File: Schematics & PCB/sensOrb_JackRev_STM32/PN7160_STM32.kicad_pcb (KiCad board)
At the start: 4 copper layers, 56.2 x 56.2 mm, 87 parts, among them J1 USB4215-03-A_REVA, J10 Conn_01x02, J11 STM32 Optional I/O, J12 Antenna_Conn, J2 Conn_01x04, J3 Conn_01x04, J4 Conn_01x04, J5 Conn_01x04, J6 Conn_01x04, J7 Conn_01x04, J8 IMU Top, J9 IMU Bottom, SW1 SW_SPST, SW2 SW_SPST, U1 PN7160A1HN/C100E, U3 STM32F411CEU6, U4 TLV75533PDBVR, U5 TPS61070DDCR, U6 TCA9548APWR, Y1 ABS07-32.768KHZ-T, Y2 TSX-3225_24.0000MF20G-AC3

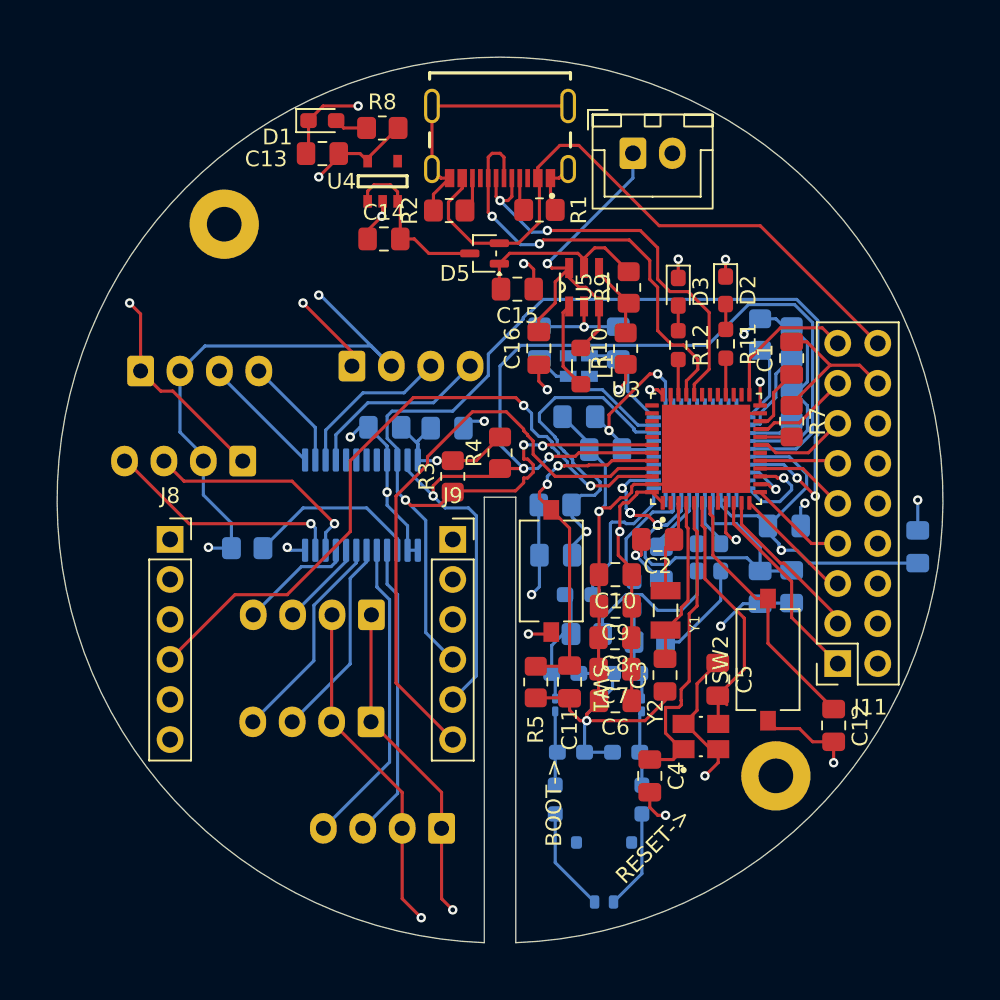
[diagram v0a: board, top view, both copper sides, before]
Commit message: Finalized PCB Layout
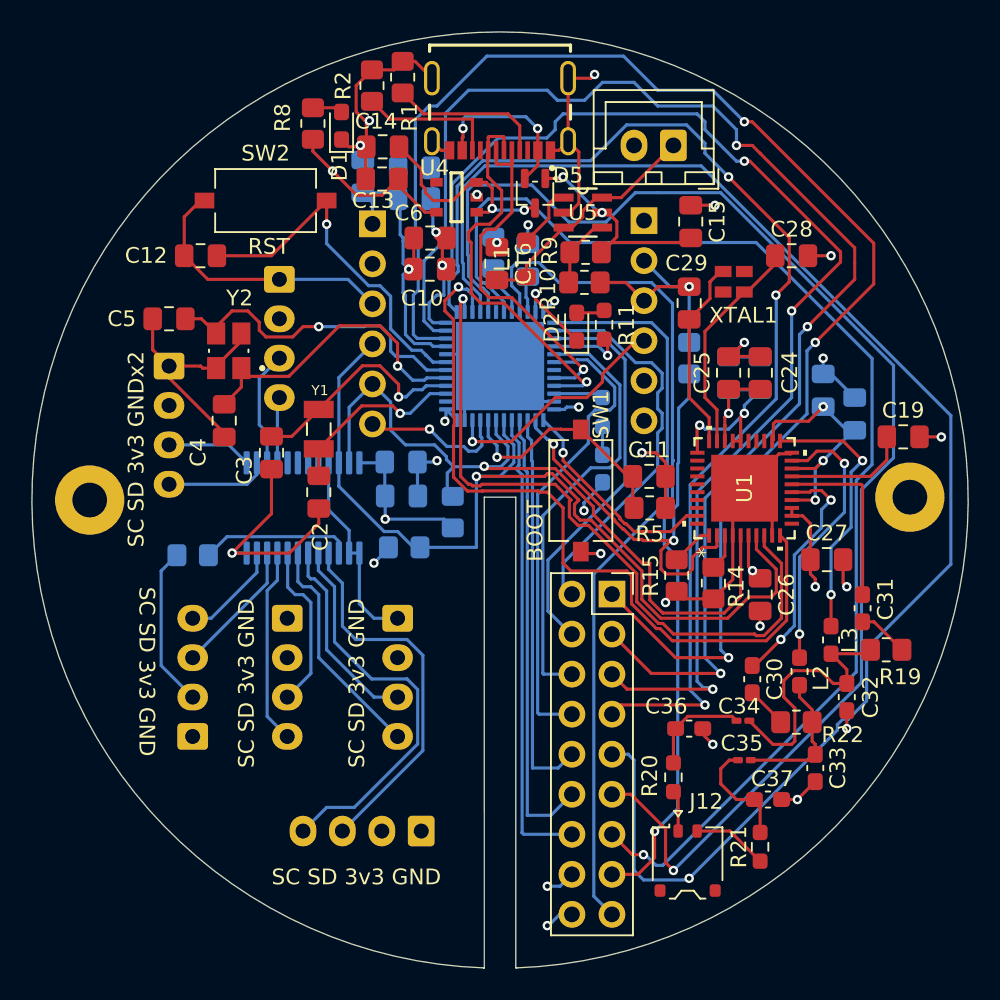
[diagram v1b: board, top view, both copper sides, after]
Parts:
- C1, C7, C8, C9, D3, J8, J9, R12, R3, R4, R7, U3: moved to B.Cu
- C19, C24, C25, C26, C27, C28, C29, C30, C31, C32, C33, C34, C35, C36, C37, J12, L2, L3, R14, R15, R19, R20, R21, R22, U1, XTAL1: moved to F.Cu
- moved C12 50.0 mm to (131.0, 84.5), turned to 180 degrees
- moved SW2 43.2 mm to (135.1, 81.0), turned to 0 degrees
- moved C5 41.7 mm to (129.0, 88.5), turned to 0 degrees
- moved Y2 38.7 mm to (132.8, 90.5), turned to 180 degrees
- moved J8 36.2 mm to (159.1, 82.3), turned to 180 degrees
- moved C4 35.2 mm to (132.5, 95.0)
- moved C7 32.4 mm to (144.6, 80.9), turned to 0 degrees
- moved C8 32.4 mm to (144.6, 78.9), turned to 0 degrees
- moved C9 31.6 mm to (141.3, 79.5), turned to 90 degrees
- moved C6 31.6 mm to (145.6, 83.4), turned to 0 degrees
- moved C3 28.7 mm to (135.5, 97.0)
- moved Y1 24.8 mm to (138.5, 95.5), turned to 90 degrees
- moved C10 22.7 mm to (145.5, 85.4), turned to 0 degrees
- moved R7 21.7 mm to (149.6, 84.3)
- moved C2 21.7 mm to (138.5, 99.5), turned to -90 degrees
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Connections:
- J11 pad 18: +5V -> +3.3V
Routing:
- net /PA6: track 5.84 -> 95.2 mm, vias 0 -> 1
- net /PA7: track 5.00 -> 86.8 mm, vias 0 -> 1
- net /PA0: track 12.9 -> 91.6 mm, vias 0 -> 3
- net /PA1: track 10.3 -> 86.9 mm, vias 0 -> 3
- net /PB1: track 5.90 -> 78.5 mm, vias 0 -> 1
- net /PA2: track 7.72 -> 80.3 mm, vias 0 -> 3
- net /PA3: track 6.27 -> 73.3 mm, vias 0 -> 3
- net +3.3V: track 142.6 -> 75.8 mm
- net /PB10: track 6.17 -> 54.0 mm, vias 0 -> 1
- net GND: track 230.5 -> 186.7 mm
- net /VEN: track 5.91 -> 49.6 mm
- net /IRQ: track 3.33 -> 44.9 mm
- net /PB12: track 9.10 -> 46.6 mm
- net +5V: track 40.8 -> 10.6 mm, vias 0 -> 2
- net /PA9: track 0.00 -> 30.1 mm
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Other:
- board size 56.2 x 56.2 mm -> 59.4 x 59.4 mm
- board text added: "3v3"
- board text added: "BOOT"
- board text added: "GND"
- board text added: "IMU BOT"
- board text added: "IMU TOP"
- board text added: "INT"
- board text added: "PA0"
- board text added: "PA1"
- board text added: "PA2"
- board text added: "PA3"
- board text added: "PA6"
- board text added: "PA7"
- board text added: "PA8"
- board text added: "PA9"
- board text added: "PB1"
- board text added: "PB10"
- board text added: "PB12"
- board text added: "PB13"
- board text added: "PB14"
- board text added: "PB3"
- board text added: "PB4"
- board text added: "PB5"
- board text added: "PN7160-STM32 Barometer-IMU Integration v1.0 Jack Cunningham - 3/31/26 OSU SIM Lab"
- board text added: "RST"
- board text added: "SC SD 3v3 GND"
- board text added: "SC SD 3v3 GNDx2"
- board text added: "SCL"
- board text added: "SDA"
- board text removed: "BOOT->"
- board text removed: "RESET->"
